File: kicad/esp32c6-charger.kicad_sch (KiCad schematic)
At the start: 21 parts, among them J1 Conn_01x06_Socket, J2 Conn_01x03_Socket, J3 Conn_Coaxial_Power, K1 G2RL-1, Q1 BC817, Q2 BC817, U1 XIAO-ESP32-C6, U2 AMS1117-5.0

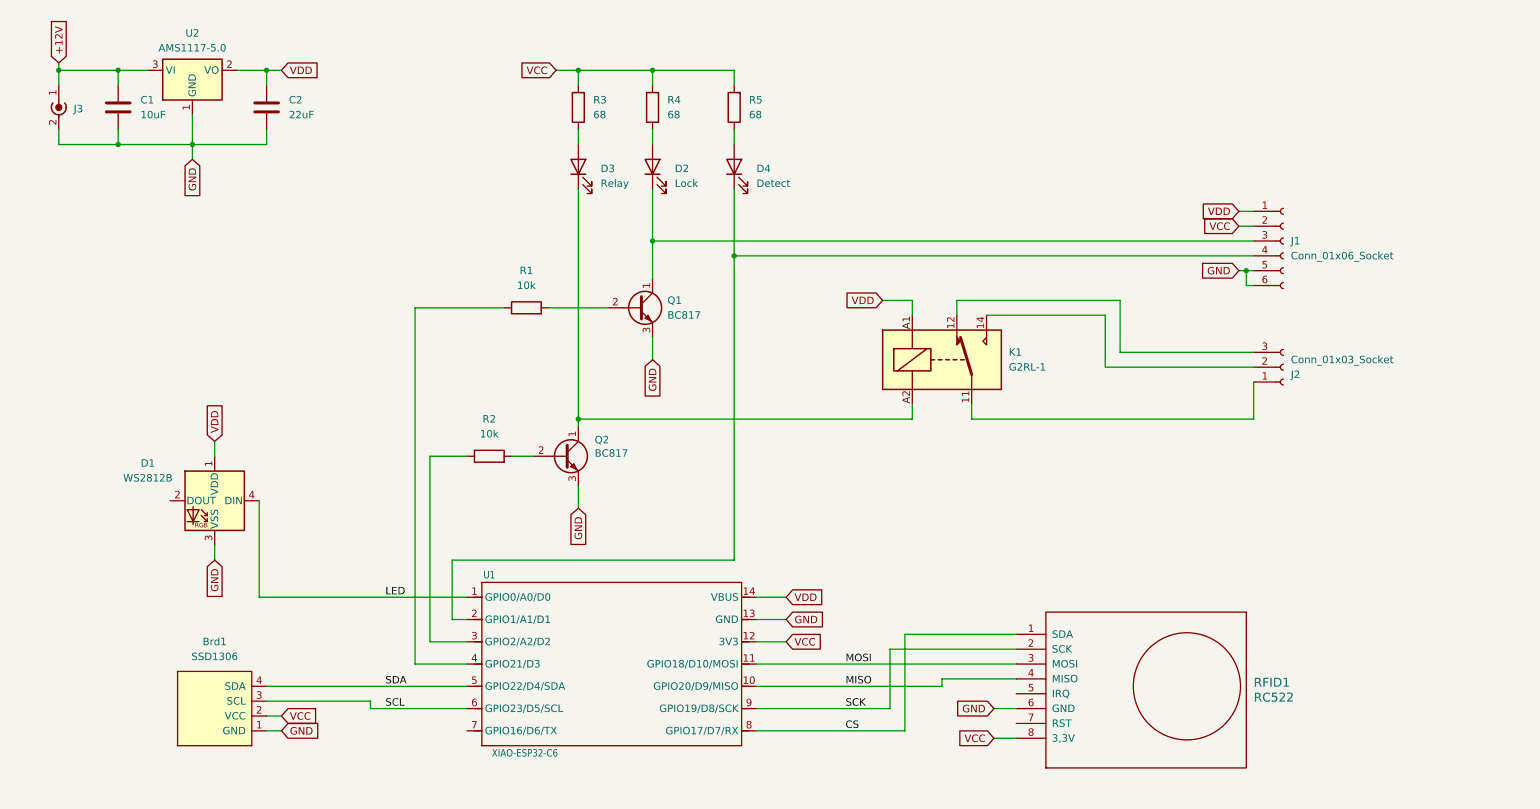
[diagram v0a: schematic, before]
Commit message: updated changes to schematic and pcb
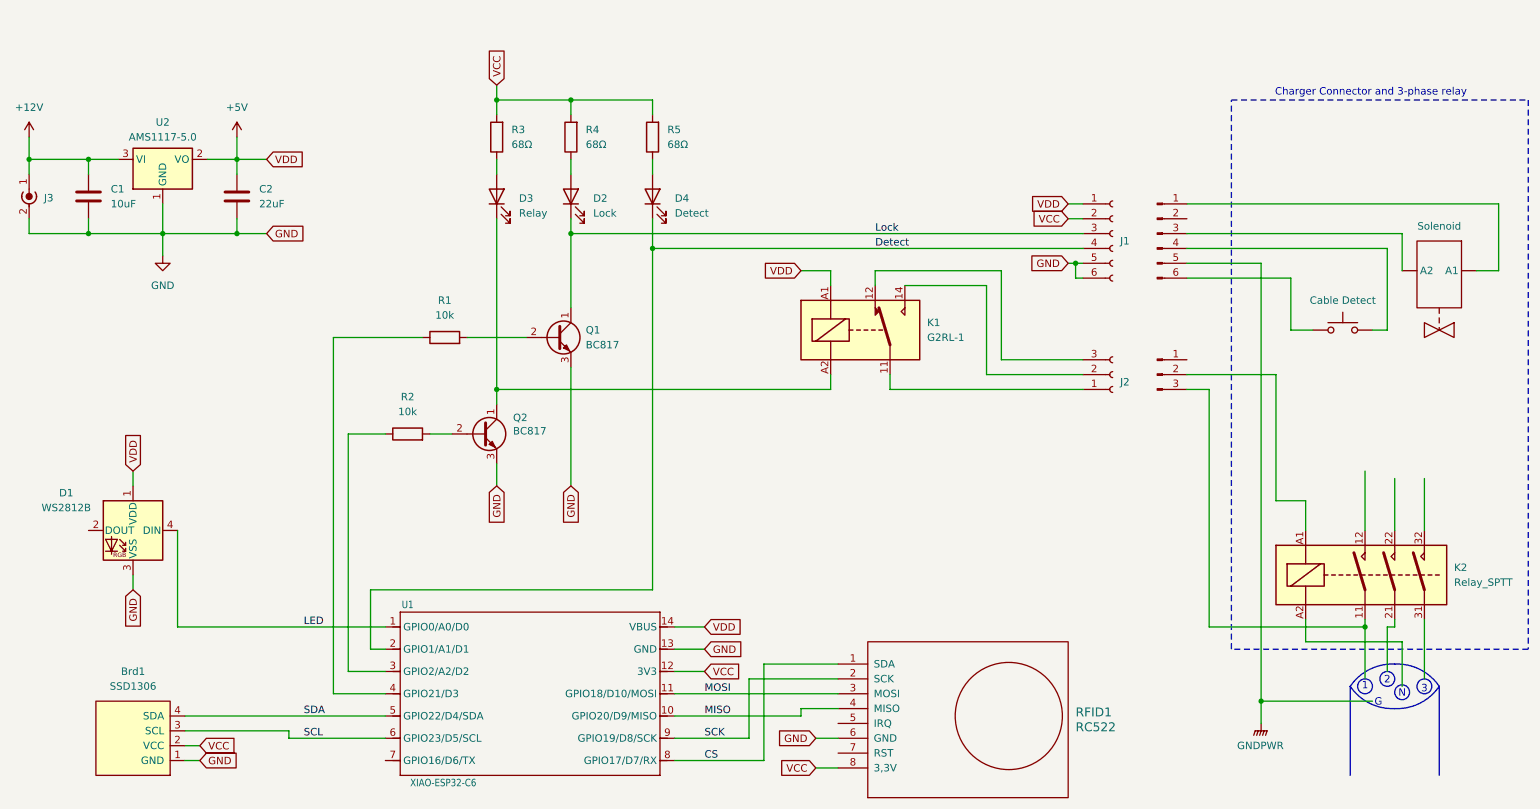
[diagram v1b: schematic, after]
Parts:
- added J4: Conn_01x06_Pin, symbol Connector:Conn_01x06_Pin
- added J5: Conn_01x03_Pin, symbol Connector:Conn_01x03_Pin
- added K2: Relay_SPTT, symbol CustomSymbols:Relay_SPTT
- added SW1: Cable Detect, symbol Switch:SW_Push
- added U3: Solenoid, symbol CustomSymbols:Solenoid
- C1, C2: footprint Capacitor_SMD:C_0805_2012Metric_Pad1.18x1.45mm_HandSolder -> Capacitor_Tantalum_SMD:CP_EIA-6032-28_Kemet-C
- J1: value Conn_01x06_Socket -> Power/Lock/Detect
- J2: value Conn_01x03_Socket -> Relay
- R3, R4, R5: value 68 -> 68Ω
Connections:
- net Lock: now reaches D2.1 (K), J1.3 (Pin_3), Q1.1 (C)
- net Detect: now reaches D4.1 (K), J1.4 (Pin_4), U1.2 (GPIO1/A1/D1)
- net VDD renamed +5V
- new net: J4.1 (Pin_1), U3. (A2)
- new net: J4.3 (Pin_3), U3. (A2)
- new net: J5.3 (Pin_3), K2.11
- new net: J5.2 (Pin_2), K2.A1
- new net: J4.6 (Pin_6), SW1.1
- new net: J4.4 (Pin_4), SW1.2
- new net GNDPWR: J4.5 (Pin_5)
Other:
- note added: "1"
- note added: "2"
- note added: "3"
- note added: "Charger Connector and 3-phase relay"
- note added: "G"
- note added: "N"
- company: (none) -> https://gertjanassies.dev/blog?category=make
- title: (none) -> ESP32-C6 EV Charger
- moved on the sheet: Brd1, C1, C2, D1, D2, D3, D4, J1, J2, J3, K1, Q1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
